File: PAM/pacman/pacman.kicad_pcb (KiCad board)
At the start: 2 copper layers, 92.7 x 66 mm, 20 parts, among them J1 Conn_01x08, J2 Conn_01x04, J6 TE Mate-N-Lok, J7 TE Mate-N-Lok, J8 TE Mate-N-Lok, J9 JST PH, K1 G2RL, K2 G5V-1, Q2 MMBT2222A

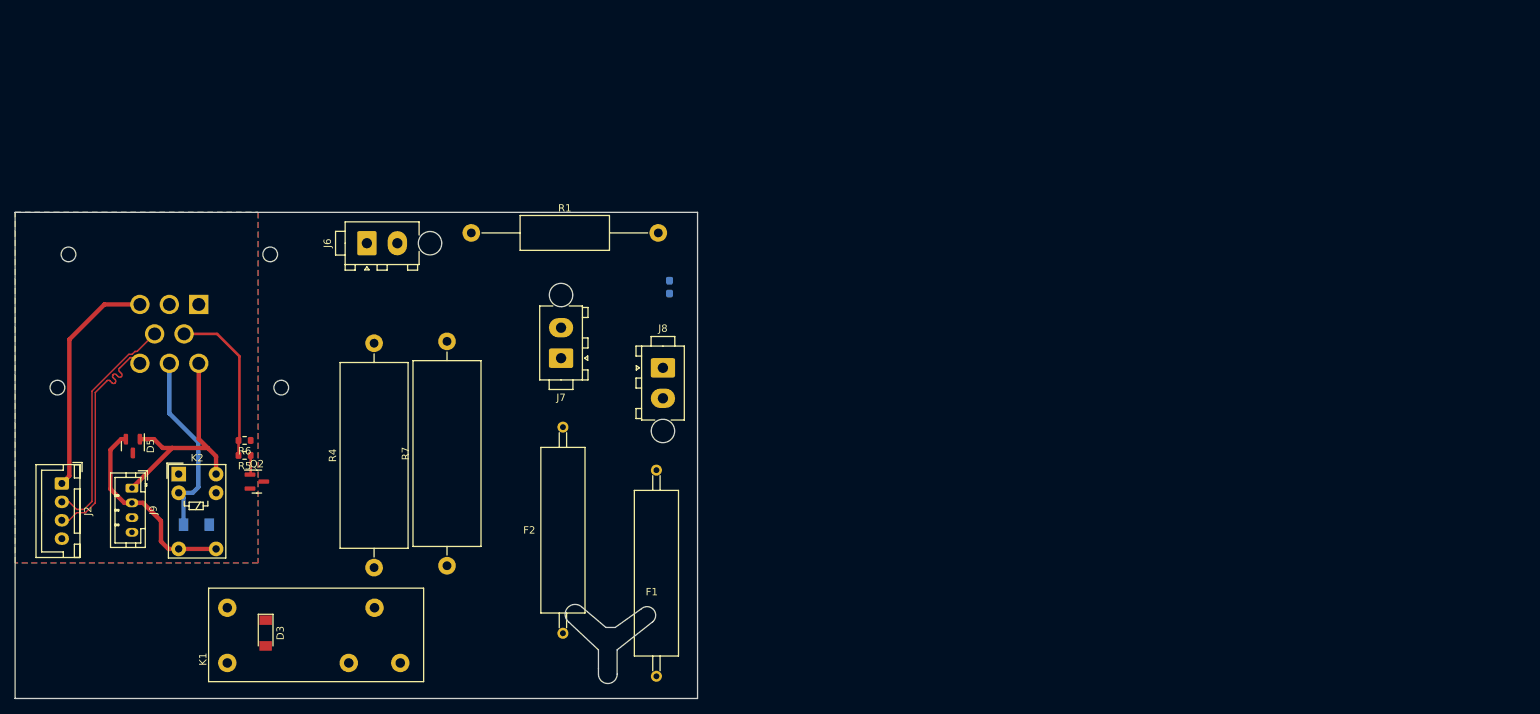
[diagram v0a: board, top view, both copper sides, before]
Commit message: DRC updating
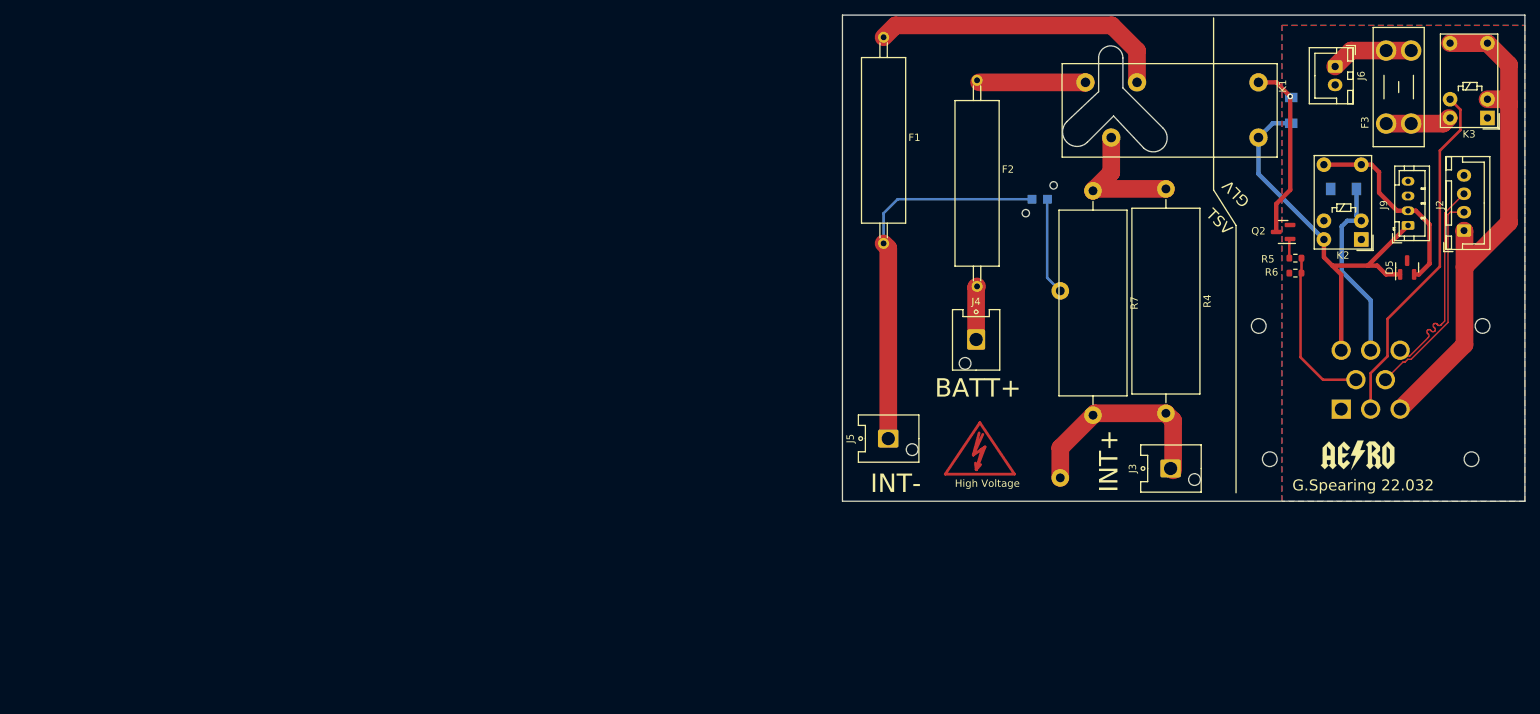
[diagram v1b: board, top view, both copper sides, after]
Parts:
- removed J7, J8: TE Mate-N-Lok, AERO_Footprints:TE_MATE-N-LOK_1-770866-x_1x02_P4.14mm_Vertical
- added F3: Fuse, AERO_Footprints:Fuseholder_Blade_Mini_Keystone_3568, F.Cu at (185.0, 64.1)
- added G***: LOGO, AERO_Footprints:AERO_Logo_10x4mm, F.Cu at (181.1, 109.2)
- added High Voltage: Symbol_HighVoltage_Type2_CopperTop_VerySmall, Symbol:Symbol_HighVoltage_Type2_CopperTop_VerySmall, F.Cu at (129.8, 109.0)
- added J3: Conn_01x01, Connector_Hirose:Hirose_DF63M-1P-3.96DSA_1x01_P3.96mm_Vertical, F.Cu at (155.7, 111.0)
- added J4: Conn_01x01, Connector_Hirose:Hirose_DF63M-1P-3.96DSA_1x01_P3.96mm_Vertical, F.Cu at (129.3, 93.5)
- added J5: Conn_01x01, Connector_Hirose:Hirose_DF63M-1P-3.96DSA_1x01_P3.96mm_Vertical, F.Cu at (117.3, 106.9)
- added K3: G5V-1, Relay_THT:Relay_SPDT_Omron_G5V-1, F.Cu at (198.7, 63.4)
- D1: footprint LED_SMD:LED_0603_1608Metric_Pad1.05x0.95mm_HandSolder -> AERO_Footprints:LPA-C011301S-x LED 0805 LIGHT PIPE SINGLE VERT SMD
- D3, R1: moved to B.Cu
- J6: value TE Mate-N-Lok -> Conn_01x02; footprint AERO_Footprints:TE_MATE-N-LOK_1-770866-x_1x02_P4.14mm_Vertical -> Connector_JST:JST_XH_B2B-XH-A_1x02_P2.50mm_Vertical
- moved J2 193.6 mm to (195.6, 78.7), turned to 90 degrees
- moved J9 177.0 mm to (188.0, 78.0), turned to 90 degrees
- moved D5 174.8 mm to (187.8, 83.7), turned to 90 degrees
- moved K2 163.8 mm to (181.6, 79.9), turned to 180 degrees
- moved J1 163.3 mm to (182.9, 98.9), turned to 0 degrees
- moved D4 162.4 mm to (179.2, 73.0), turned to 180 degrees
- moved D3 156.4 mm to (172.1, 62.4), turned to 90 degrees
- moved R5 145.2 mm to (172.7, 82.4), turned to 0 degrees
- moved R6 144.5 mm to (172.7, 84.5), turned to 0 degrees
- moved Q2 143.5 mm to (171.0, 78.9), turned to 180 degrees
- moved K1 135.0 mm to (154.9, 62.4), turned to 180 degrees
- moved J6 133.7 mm to (178.1, 56.4), turned to -90 degrees
- moved R4 119.2 mm to (155.1, 73.0), turned to -90 degrees
- moved R7 101.5 mm to (145.2, 73.3), turned to -90 degrees
- moved R1 86.7 mm to (140.7, 112.3), turned to 90 degrees
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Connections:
- J1 pad 2: GND -> /BMS_FAN
- J6 pad 1: /INT+ -> Net-(F3-Pad2)
- J6 pad 2: /INT+ -> GND
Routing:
- net /INT-: track 0.00 -> 52.0 mm
- net /BMS_FAN: track 0.00 -> 47.7 mm
- net Net-(F1-Pad1): track 0.00 -> 40.8 mm
- net +12V: track 31.5 -> 70.3 mm
- net /INT+: track 0.00 -> 28.5 mm
- net Net-(D3-Pad2): track 0.00 -> 24.3 mm, vias 0 -> 1
- net /AIR_B-: track 33.4 -> 56.2 mm
- net Net-(K1-Pad5): track 0.00 -> 18.3 mm
- net Net-(F2-Pad1): track 0.00 -> 14.6 mm
- net Net-(D1-Pad2): track 0.00 -> 13.0 mm
- net Net-(F3-Pad2): track 0.00 -> 11.2 mm
- net /FAN_OUT: track 0.00 -> 8.82 mm
- net /B+: track 0.00 -> 7.26 mm
- net /BMS_CAN+: track 31.7 -> 28.7 mm
- net /BMS_CAN-: track 31.7 -> 28.7 mm
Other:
- outline, holes or cut-outs redrawn
- board text added: "BATT+"
- board text added: "G.Spearing 22.032"
- board text added: "GLV"
- board text added: "INT+"
- board text added: "INT-"
- board text added: "TSV"
